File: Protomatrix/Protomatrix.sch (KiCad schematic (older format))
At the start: 141 parts, among them J1 Conn_01x21_Female

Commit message: routing & more
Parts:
- J1: value Conn_01x21_Female -> Conn_01x18_Female; footprint Connector_PinHeader_2.54mm:PinHeader_1x21_P2.54mm_Horizontal -> Connector_PinHeader_2.54mm:PinHeader_1x18_P2.54mm_Vertical; symbol Connector:Conn_01x21_Female -> Connector:Conn_01x18_Female
- MX-LShift1: renamed from MX-RShift1; footprint MX_Only:MXOnly-2.75U-NoLED -> MX_Only:MXOnly-2.25U-NoLED
- MX-RShift1: renamed from MX-Lshift1; footprint MX_Only:MXOnly-2.25U-NoLED -> MX_Only:MXOnly-2.75U-NoLED
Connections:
- net Col10: now also MX-PgDn1.1 (COL); no longer MX-RAlt1.1 (COL)
- net Col11: now also MX-PgUp1.1 (COL), MX-RShift1.1 (COL); no longer MX-RSys1.1 (COL)
- net Col12: no longer MX-RCtrl1.1 (COL), MX-RShift1.1 (COL)
- net Col13: now also MX-Del1.1 (COL), MX-Hm1.1 (COL), MX-Ins1.1 (COL)
- net Col3: now also MX-Spc1.1 (COL)
- net Col4: now also MX-RAlt1.1 (COL)
- net Col5: now also MX-RSys1.1 (COL); no longer MX-Spc1.1 (COL)
- net Col6: now also MX-RCtrl1.1 (COL)
- net Col7: now also MX-Left1.1 (COL)
- net Col8: now also MX-Down1.1 (COL)
- net Col9: now also MX-Right1.1 (COL)
- net Row0: no longer D15.1 (K), D16.1 (K), D17.1 (K)
- net Row1: no longer D31.1 (K), D32.1 (K), D33.1 (K)
- net Row2: now also D15.1 (K)
- net Row3: now also D31.1 (K)
- net Row4: now also D16.1 (K), D17.1 (K), D32.1 (K), D33.1 (K)
- removed net Col14: J1.19 (Pin_19), MX-Del1.1 (COL), MX-Ins1.1 (COL), MX-Left1.1 (COL)
- removed net Col15: J1.20 (Pin_20), MX-Down1.1 (COL), MX-Hm1.1 (COL), MX-Up1.1 (COL), MX-end1.1 (COL)
- removed net Col16: J1.21 (Pin_21), MX-PgDn1.1 (COL), MX-PgUp1.1 (COL), MX-Right1.1 (COL)
- new net: MX-Up1.1 (COL), MX-end1.1 (COL)
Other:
- moved on the sheet: D15, D16, D17, D31, D32, D33, D59, D60, D64, D65, D66, D67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

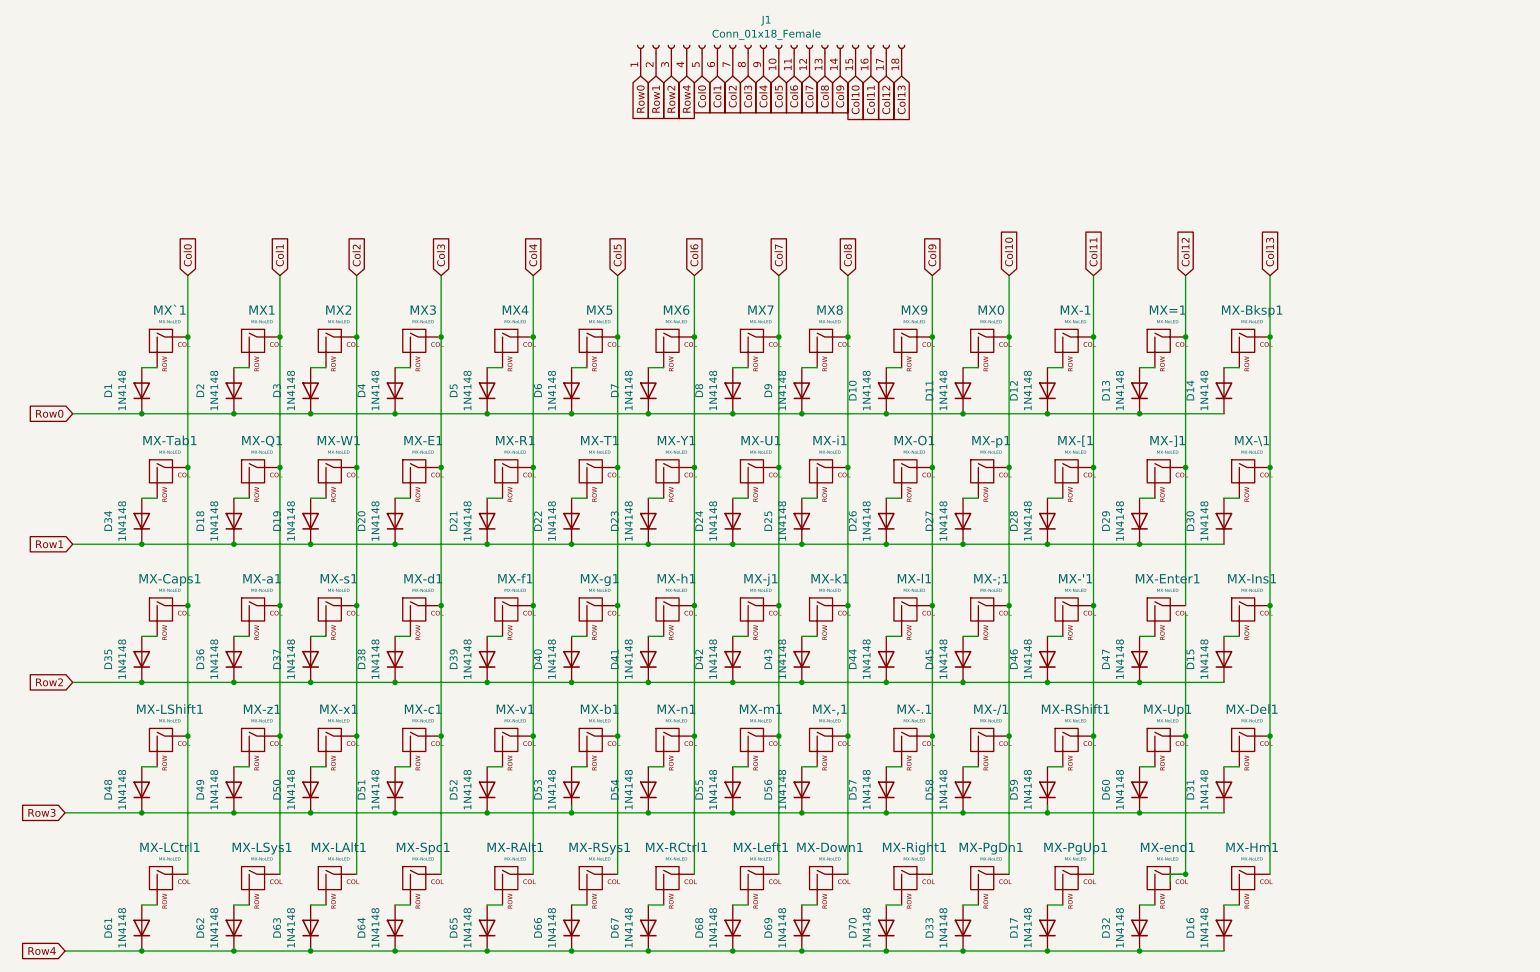
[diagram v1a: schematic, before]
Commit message: The Routing Continues
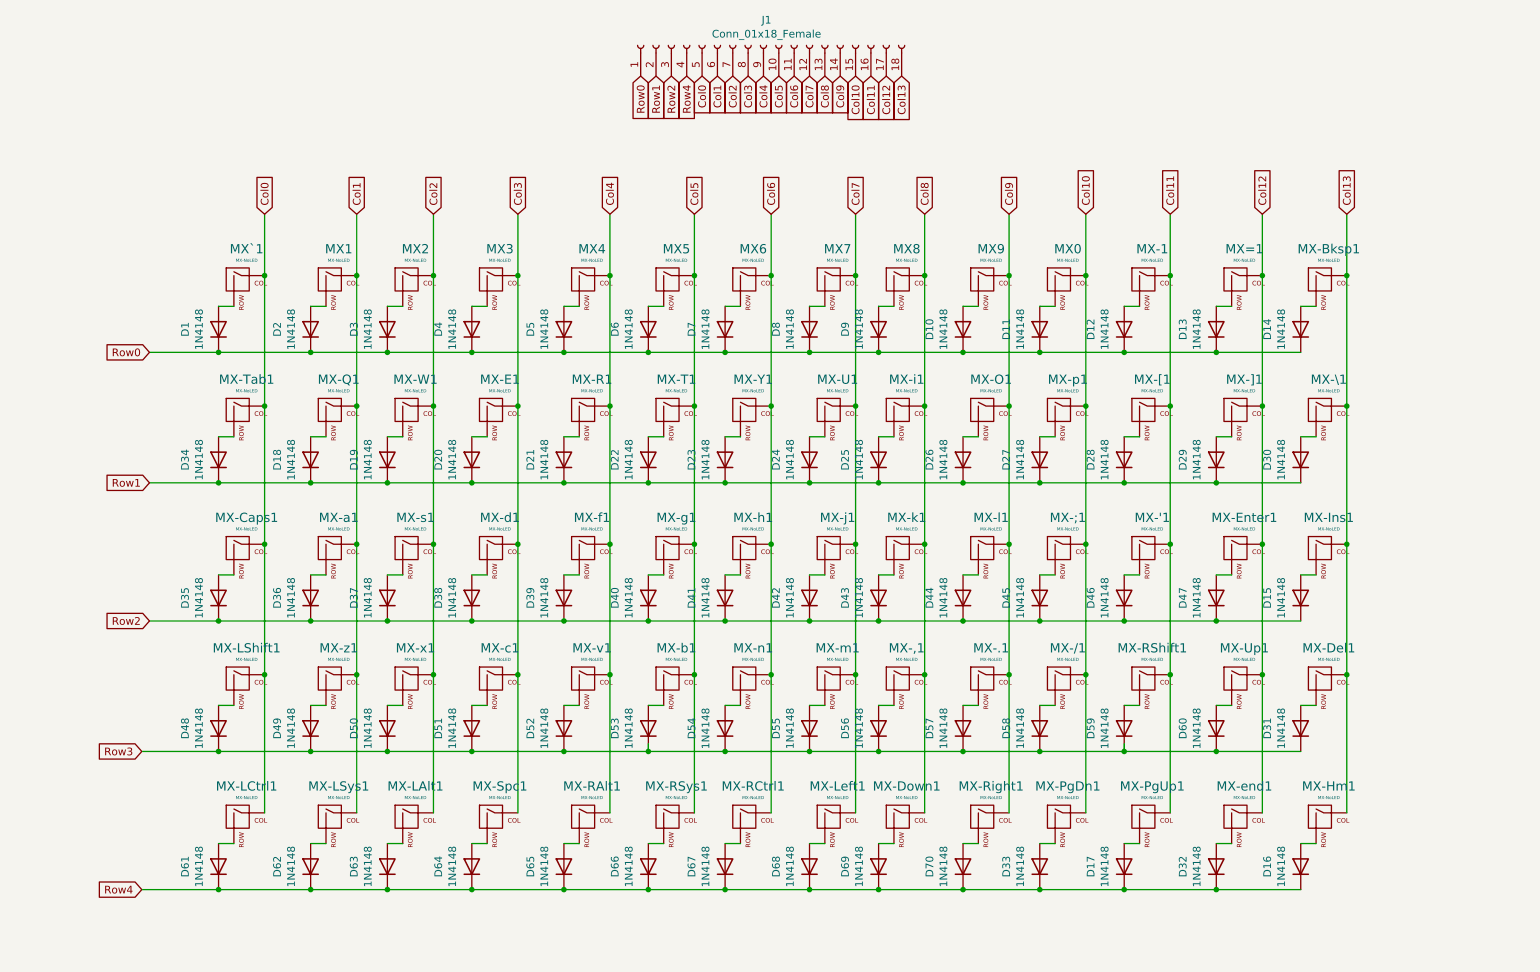
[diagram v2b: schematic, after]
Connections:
- net Col12: now also MX-Up1.1 (COL), MX-end1.1 (COL)
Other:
- moved on the sheet: D1, D10, D11, D12, D13, D14, D15, D16, D17, D18, D19, D2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

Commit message: Version 0.1 Complete
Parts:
- J1: value Conn_01x18_Female -> Conn_01x20_Female; footprint Connector_PinHeader_2.54mm:PinHeader_1x18_P2.54mm_Vertical -> Connector_PinHeader_2.54mm:PinHeader_1x20_P2.54mm_Vertical; symbol Connector:Conn_01x18_Female -> Connector:Conn_01x20_Female
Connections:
- net Col0: now also J1.7 (Pin_7); no longer J1.5 (Pin_5)
- net Col1: now also J1.8 (Pin_8); no longer J1.6 (Pin_6)
- net Col10: now also J1.17 (Pin_17); no longer J1.15 (Pin_15)
- net Col11: now also J1.18 (Pin_18); no longer J1.16 (Pin_16)
- net Col12: now also J1.19 (Pin_19); no longer J1.17 (Pin_17)
- net Col13: now also J1.20 (Pin_20); no longer J1.18 (Pin_18)
- net Col2: now also J1.9 (Pin_9); no longer J1.7 (Pin_7)
- net Col3: now also J1.10 (Pin_10); no longer J1.8 (Pin_8)
- net Col4: now also J1.11 (Pin_11); no longer J1.9 (Pin_9)
- net Col5: now also J1.12 (Pin_12); no longer J1.10 (Pin_10)
- net Col6: now also J1.13 (Pin_13); no longer J1.11 (Pin_11)
- net Col7: now also J1.14 (Pin_14); no longer J1.12 (Pin_12)
- net Col8: now also J1.15 (Pin_15); no longer J1.13 (Pin_13)
- net Col9: now also J1.16 (Pin_16); no longer J1.14 (Pin_14)
- net Row3: now also J1.4 (Pin_4)
- net Row4: now also J1.5 (Pin_5); no longer J1.4 (Pin_4)
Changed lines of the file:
@@
 $EndDescr
 $Comp
-L Connector:Conn_01x18_Female J1
+L Connector:Conn_01x20_Female J1
 U 1 1 5FBC2DAD
 P 5650 1050
 F 0 "J1" V 5815 1030 50  0000 C CNN
-F 1 "Conn_01x18_Female" V 5724 1030 50  0000 C CNN
-F 2 "Connector_PinHeader_2.54mm:PinHeader_1x18_P2.54mm_Vertical" H 5650 1050 50  0001 C CNN
+F 1 "Conn_01x20_Female" V 5724 1030 50  0000 C CNN
+F 2 "Connector_PinHeader_2.54mm:PinHeader_1x20_P2.54mm_Vertical" H 5650 1050 50  0001 C CNN
 F 3 "~" H 5650 1050 50  0001 C CNN
 	1    5650 1050
@@
 Text GLabel 9450 2150 1    50   Input ~ 0
 Col13
-Text GLabel 5250 1250 3    50   Input ~ 0
+Text GLabel 5350 1250 3    50   Input ~ 0
 Col0
-Text GLabel 5350 1250 3    50   Input ~ 0
+Text GLabel 5450 1250 3    50   Input ~ 0
 Col1
-Text GLabel 5450 1250 3    50   Input ~ 0
+Text GLabel 5550 1250 3    50   Input ~ 0
 Col2
-Text GLabel 5550 1250 3    50   Input ~ 0
+Text GLabel 5650 1250 3    50   Input ~ 0
 Col3
-Text GLabel 5650 1250 3    50   Input ~ 0
+Text GLabel 5750 1250 3    50   Input ~ 0
 Col4
-Text GLabel 5750 1250 3    50   Input ~ 0
+Text GLabel 5850 1250 3    50   Input ~ 0
 Col5
-Text GLabel 5850 1250 3    50   Input ~ 0
+Text GLabel 5950 1250 3    50   Input ~ 0
 Col6
-Text GLabel 5950 1250 3    50   Input ~ 0
+Text GLabel 6050 1250 3    50   Input ~ 0
 Col7
-Text GLabel 6050 1250 3    50   Input ~ 0
+Text GLabel 6150 1250 3    50   Input ~ 0
 Col8
-Text GLabel 6150 1250 3    50   Input ~ 0
+Text GLabel 6250 1250 3    50   Input ~ 0
 Col9
-Text GLabel 6250 1250 3    50   Input ~ 0
+Text GLabel 6350 1250 3    50   Input ~ 0
 Col10
-Text GLabel 6350 1250 3    50   Input ~ 0
+Text GLabel 6450 1250 3    50   Input ~ 0
 Col11
-Text GLabel 6450 1250 3    50   Input ~ 0
+Text GLabel 6550 1250 3    50   Input ~ 0
 Col12
-Text GLabel 6550 1250 3    50   Input ~ 0
+Text GLabel 6650 1250 3    50   Input ~ 0
 Col13
+Text GLabel 4750 1250 3    50   Input ~ 0
+Row0
 Text GLabel 4850 1250 3    50   Input ~ 0
-Row0
+Row1
 Text GLabel 4950 1250 3    50   Input ~ 0
-Row1
-Text GLabel 5050 1250 3    50   Input ~ 0
 Row2
 Text GLabel 5150 1250 3    50   Input ~ 0
@@
 	8900 6050 8900 5150
 Connection ~ 8900 5150
+Text GLabel 5050 1250 3    50   Input ~ 0
+Row3
 $EndSCHEMATC
